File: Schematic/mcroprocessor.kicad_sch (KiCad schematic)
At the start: 11 parts, among them SW1 SW_Push, U1 STM32F091RCT6

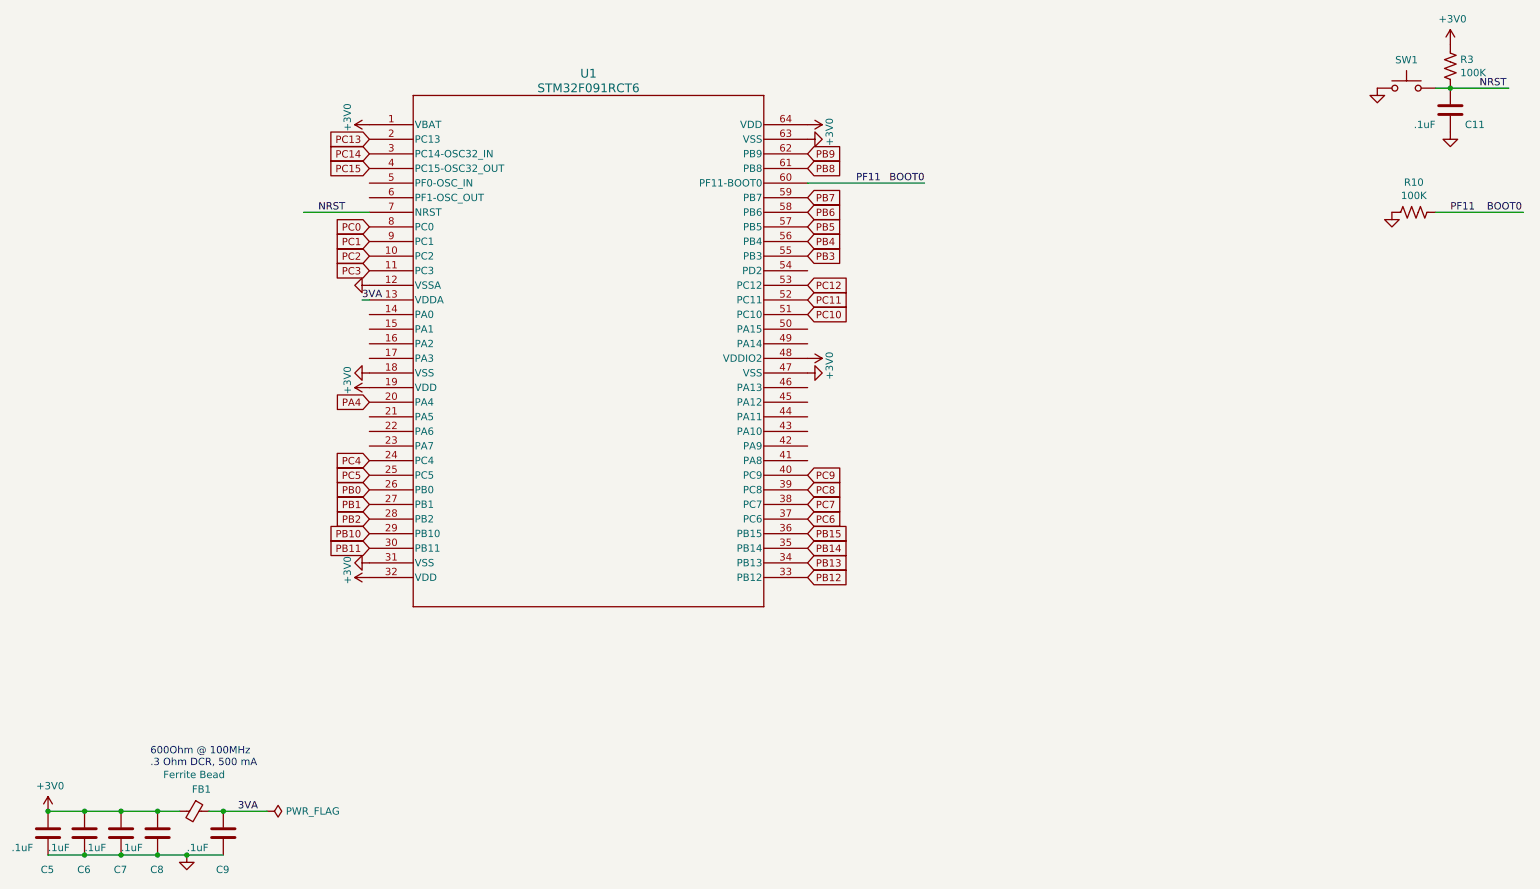
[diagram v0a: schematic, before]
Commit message: initial CB design
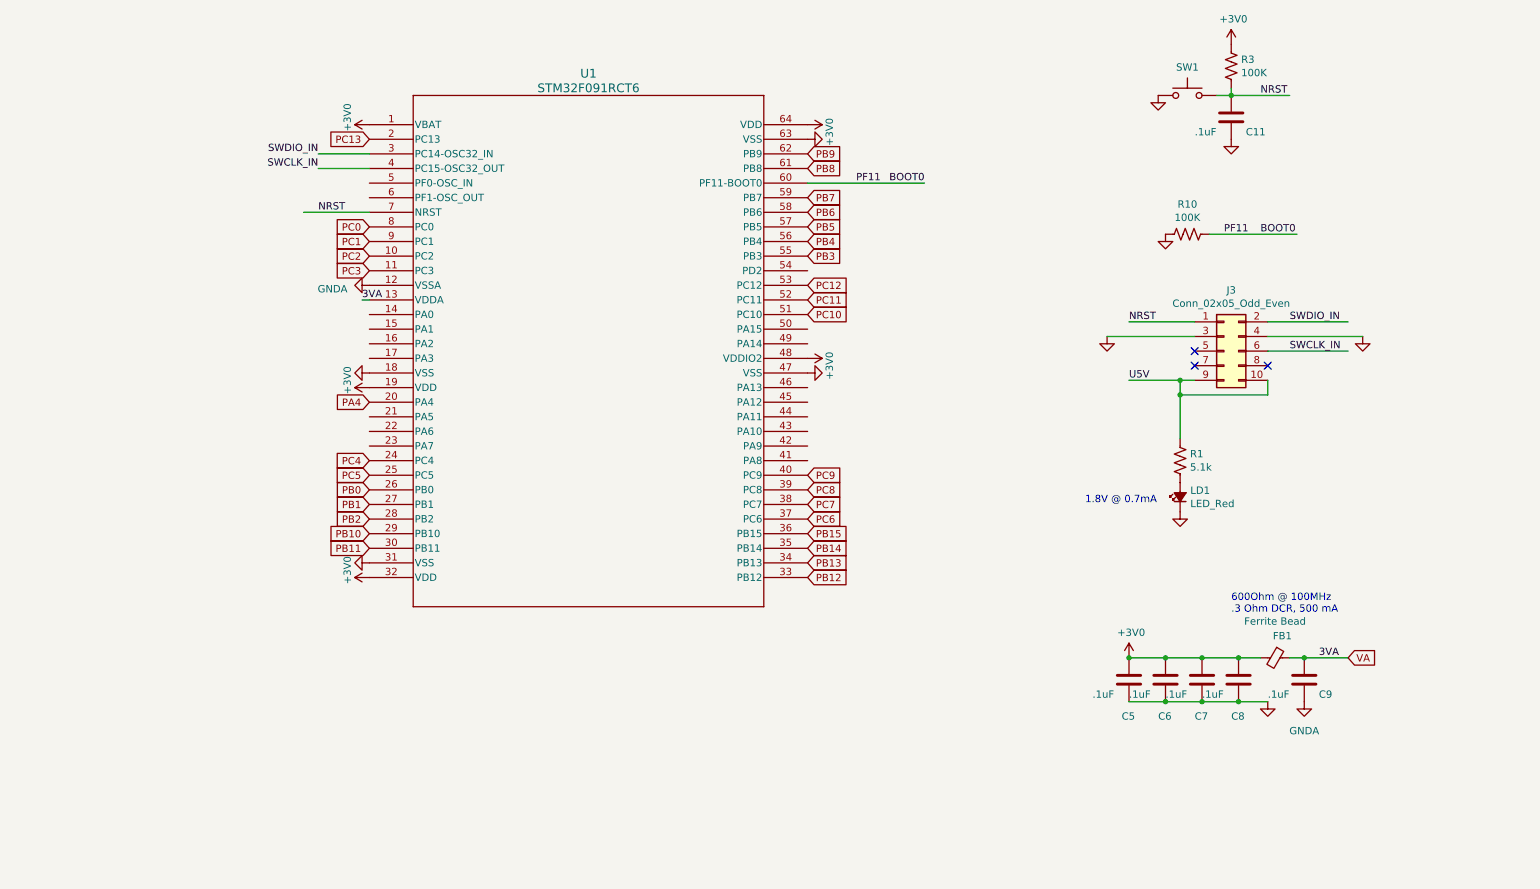
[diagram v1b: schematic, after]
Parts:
- added J3: Conn_02x05_Odd_Even, Connector_IDC:IDC-Header_2x05_P2.54mm_Vertical, symbol Connector_Generic:Conn_02x05_Odd_Even
- added LD1: LED_Red, LED_THT:LED_D5.0mm, symbol stm32f091-rescue:LED_Small_ALT-Device
- added R1: 5.1k, Resistor_SMD:R_1206_3216Metric_Pad1.30x1.75mm_HandSolder, symbol Device:R_US
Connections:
- net GND: now also J3.3 (Pin_3), J3.4 (Pin_4), LD1.1 (K); no longer C9.2, U1.12 (VSSA)
- net NRST: now also J3.1 (Pin_1)
- net 3VA renamed VA
- net PC14 renamed SWDIO_IN
- net SWDIO_IN: now also J3.2 (Pin_2)
- net PC15 renamed SWCLK_IN
- net SWCLK_IN: now also J3.6 (Pin_6)
- new net: LD1.2 (A), R1.2
- new net GNDA: C9.2, U1.12 (VSSA)
- new net U5V: J3.10 (Pin_10), J3.9 (Pin_9), R1.1
- no-connect marks 0 -> 3
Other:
- note added: "1.8V @ 0.7mA"
- moved on the sheet: C11, C5, C6, C7, C8, C9, FB1, R10, R3, SW1
